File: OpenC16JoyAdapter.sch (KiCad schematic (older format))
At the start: 8 parts, among them J1 DB9_MALE, J2 TO_C16_MINI_DIN_8, SW1 PIN5_POWER, U1 74LS244

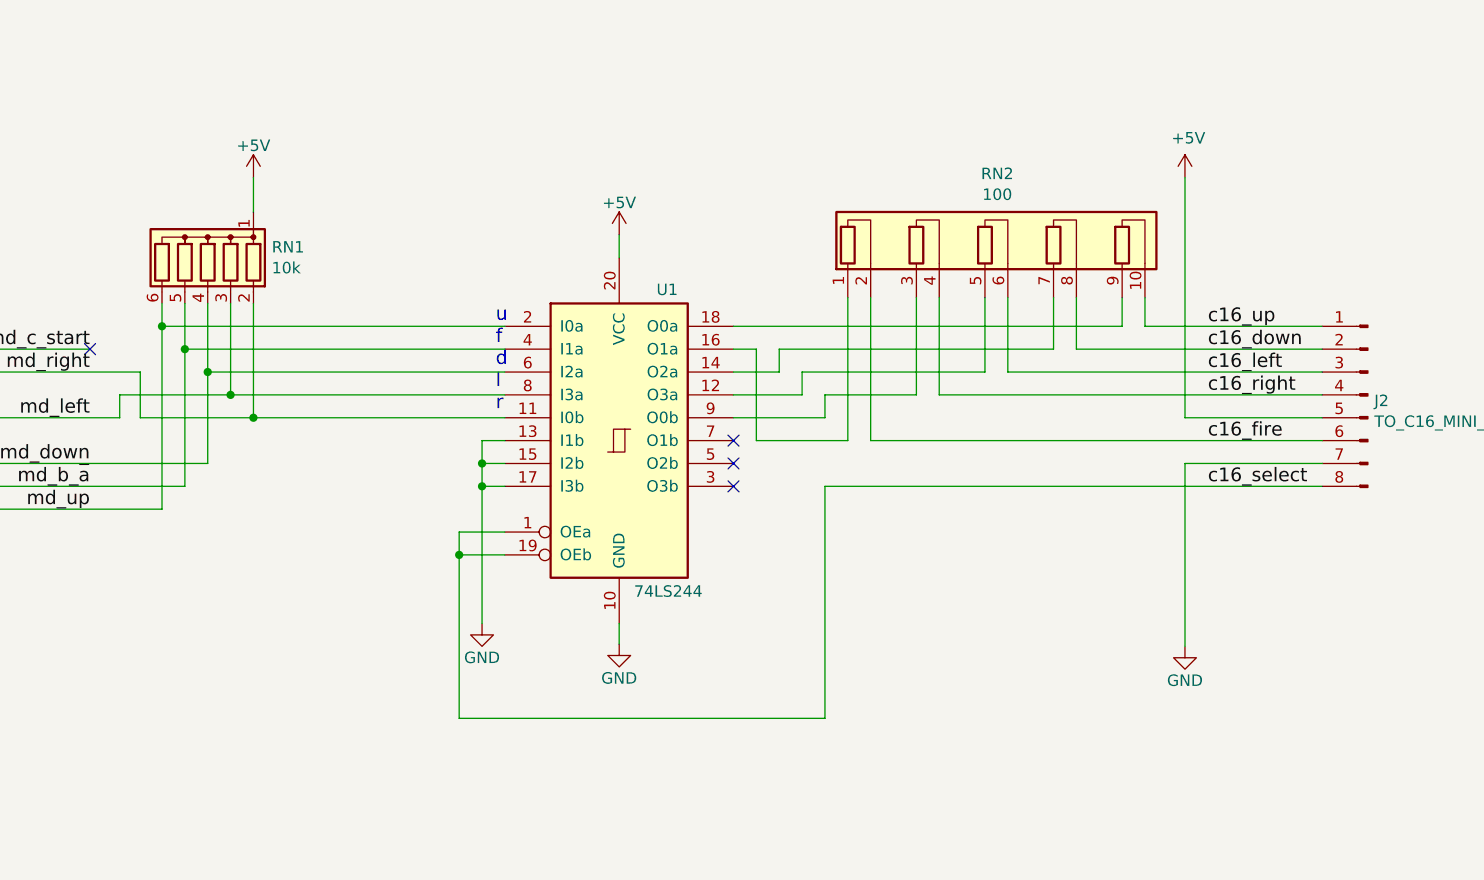
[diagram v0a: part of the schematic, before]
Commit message: Minor changes
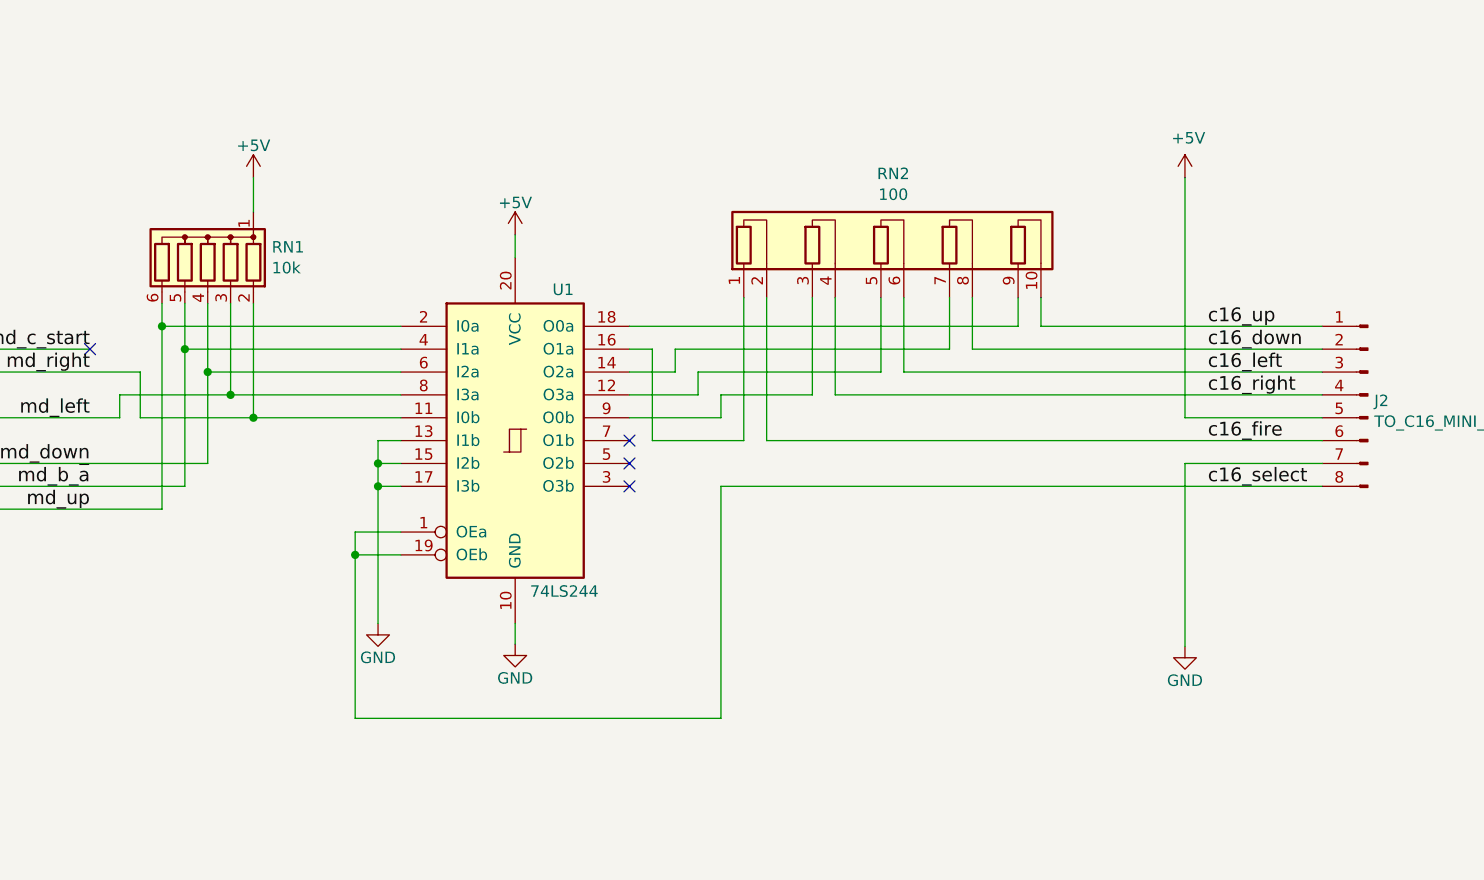
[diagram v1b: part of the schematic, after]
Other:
- note removed: "u\nf\nd\nl\nr"
- moved on the sheet: RN2, U1
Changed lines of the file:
@@
 Comp "SukkoPera"
 Comment1 "http://www.commodore.ca/manuals/funet/cbm/documents/projects/interfaces/plus4joy/plus4joy.html"
-Comment2 "Based on work by Levente Hársfalvi"
+Comment2 "Based on work by Levente Hársfalvi (TLC)"
 Comment3 "Licensed under CERN OHL v.1.2"
 Comment4 ""
@@
 L power:GND #PWR02
 U 1 1 5964022D
-P 4750 4600
-F 0 "#PWR02" H 4750 4350 50  0001 C CNN
-F 1 "GND" H 4750 4450 50  0000 C CNN
-F 2 "" H 4750 4600 50  0000 C CNN
-F 3 "" H 4750 4600 50  0000 C CNN
-	1    4750 4600
+P 4295 4600
+F 0 "#PWR02" H 4295 4350 50  0001 C CNN
+F 1 "GND" H 4295 4450 50  0000 C CNN
+F 2 "" H 4295 4600 50  0000 C CNN
+F 3 "" H 4295 4600 50  0000 C CNN
+	1    4295 4600
 	1    0    0    -1
 $EndComp
@@
 $EndComp
 Wire Wire Line
-	4750 3900 4850 3900
-Wire Wire Line
-	4650 4200 4850 4200
-Wire Wire Line
-	4650 4200 4650 4300
-Wire Wire Line
-	4850 4300 4650 4300
-Connection ~ 4650 4300
+	4295 3900 4395 3900
+Wire Wire Line
+	4195 4200 4395 4200
+Wire Wire Line
+	4195 4200 4195 4300
+Wire Wire Line
+	4395 4300 4195 4300
+Connection ~ 4195 4300
 Wire Wire Line
 	2460 2615 2460 2565
 Wire Wire Line
-	4750 3800 4850 3800
-Wire Wire Line
-	4750 3800 4750 3900
-Connection ~ 4750 3900
-Connection ~ 4750 4000
+	4295 3800 4395 3800
+Wire Wire Line
+	4295 3800 4295 3900
+Connection ~ 4295 3900
+Connection ~ 4295 4000
 Wire Wire Line
 	10375 3900 10375 3750
@@
 	3450 3200 3450 3400
 Wire Wire Line
-	4750 3900 4750 4000
-Wire Wire Line
-	4750 4000 4750 4600
-Wire Wire Line
-	4750 4000 4850 4000
-Wire Wire Line
-	3350 3300 4850 3300
-Wire Wire Line
-	3450 3400 4850 3400
+	4295 3900 4295 4000
+Wire Wire Line
+	4295 4000 4295 4600
+Wire Wire Line
+	4295 4000 4395 4000
+Wire Wire Line
+	3350 3300 4395 3300
+Wire Wire Line
+	3450 3400 4395 3400
 Wire Wire Line
 	3750 2650 3750 2800
@@
 $EndComp
 Wire Wire Line
-	6350 3800 6350 3175
-Wire Wire Line
-	6450 3800 6450 3175
-Wire Wire Line
-	6650 3600 6650 3175
-Wire Wire Line
-	6750 3600 6750 3175
-Wire Wire Line
-	6950 3500 6950 3175
-Wire Wire Line
-	7050 3500 7050 3175
-Wire Wire Line
-	7250 3400 6050 3400
-Wire Wire Line
-	7250 3175 7250 3400
-Wire Wire Line
-	7350 3175 7350 3400
-Wire Wire Line
-	7550 3300 7550 3175
-Wire Wire Line
-	7650 3175 7650 3300
-Wire Wire Line
-	5350 3000 5350 2900
-Wire Wire Line
-	5950 3800 6350 3800
-Wire Wire Line
-	5950 3400 5950 3800
-Wire Wire Line
-	5850 3400 5950 3400
-Wire Wire Line
-	6250 3600 6650 3600
-Wire Wire Line
-	6250 3600 6250 3700
-Wire Wire Line
-	6250 3700 5850 3700
-Wire Wire Line
-	6150 3500 6950 3500
-Wire Wire Line
-	6150 3600 6150 3500
-Wire Wire Line
-	5850 3600 6150 3600
-Wire Wire Line
-	6050 3500 6050 3400
-Wire Wire Line
-	5850 3500 6050 3500
-Wire Wire Line
-	5850 3300 7550 3300
-Wire Wire Line
-	6250 4000 8425 4000
+	5895 3800 5895 3175
+Wire Wire Line
+	5995 3800 5995 3175
+Wire Wire Line
+	6195 3600 6195 3175
+Wire Wire Line
+	6295 3600 6295 3175
+Wire Wire Line
+	6495 3500 6495 3175
+Wire Wire Line
+	6595 3500 6595 3175
+Wire Wire Line
+	6795 3400 5595 3400
+Wire Wire Line
+	6795 3175 6795 3400
+Wire Wire Line
+	6895 3175 6895 3400
+Wire Wire Line
+	7095 3300 7095 3175
+Wire Wire Line
+	7195 3175 7195 3300
+Wire Wire Line
+	4895 3000 4895 2900
+Wire Wire Line
+	5495 3800 5895 3800
+Wire Wire Line
+	5495 3400 5495 3800
+Wire Wire Line
+	5395 3400 5495 3400
+Wire Wire Line
+	5795 3600 6195 3600
+Wire Wire Line
+	5795 3600 5795 3700
+Wire Wire Line
+	5795 3700 5395 3700
+Wire Wire Line
+	5695 3500 6495 3500
+Wire Wire Line
+	5695 3600 5695 3500
+Wire Wire Line
+	5395 3600 5695 3600
+Wire Wire Line
+	5595 3500 5595 3400
+Wire Wire Line
+	5395 3500 5595 3500
+Wire Wire Line
+	5395 3300 7095 3300
+Wire Wire Line
+	5795 4000 8425 4000
 Wire Wire Line
 	7825 3900 7825 4700
@@
 	8425 3900 7825 3900
 Wire Wire Line
-	6450 3800 8425 3800
+	5995 3800 8425 3800
 Wire Wire Line
 	7825 3700 7825 2650
@@
 	8425 3700 7825 3700
 Wire Wire Line
-	6750 3600 8425 3600
-Wire Wire Line
-	7050 3500 8425 3500
-Wire Wire Line
-	7350 3400 8425 3400
-Wire Wire Line
-	7650 3300 8425 3300
+	6295 3600 8425 3600
+Wire Wire Line
+	6595 3500 8425 3500
+Wire Wire Line
+	6895 3400 8425 3400
+Wire Wire Line
+	7195 3300 8425 3300
 $Comp
 L power:+5V #PWR08
 U 1 1 596A3F1E
-P 5350 2900
-F 0 "#PWR08" H 5350 2750 50  0001 C CNN
-F 1 "+5V" H 5350 3040 50  0000 C CNN
-F 2 "" H 5350 2900 50  0000 C CNN
-F 3 "" H 5350 2900 50  0000 C CNN
-	1    5350 2900
-	1    0    0    -1
-$EndComp
-NoConn ~ 5850 4000
-NoConn ~ 5850 3900
-NoConn ~ 5850 3800
+P 4895 2900
+F 0 "#PWR08" H 4895 2750 50  0001 C CNN
+F 1 "+5V" H 4895 3040 50  0000 C CNN
+F 2 "" H 4895 2900 50  0000 C CNN
+F 3 "" H 4895 2900 50  0000 C CNN
+	1    4895 2900
+	1    0    0    -1
+$EndComp
+NoConn ~ 5395 4000
+NoConn ~ 5395 3900
+NoConn ~ 5395 3800
 Text Label 7925 4000 0    60   ~ 0
 c16_select
@@
 L 74xx:74LS244 U1
 U 1 1 65B63CCD
-P 5350 3800
-F 0 "U1" H 5560 4460 50  0000 C CNN
-F 1 "74LS244" H 5565 3140 50  0000 C CNN
-F 2 "Package_DIP:DIP-20_W7.62mm_Socket_LongPads" H 5350 3800 50  0001 C CNN
-F 3 "http://www.ti.com/lit/ds/symlink/sn74ls244.pdf" H 5350 3800 50  0001 C CNN
-	1    5350 3800
-	1    0    0    -1
-$EndComp
-Wire Wire Line
-	5350 4600 5350 4690
+P 4895 3800
+F 0 "U1" H 5105 4460 50  0000 C CNN
+F 1 "74LS244" H 5110 3140 50  0000 C CNN
+F 2 "Package_DIP:DIP-20_W7.62mm_Socket_LongPads" H 4895 3800 50  0001 C CNN
+F 3 "http://www.ti.com/lit/ds/symlink/sn74ls244.pdf" H 4895 3800 50  0001 C CNN
+	1    4895 3800
+	1    0    0    -1
+$EndComp
+Wire Wire Line
+	4895 4600 4895 4690
 $Comp
 L power:GND #PWR0103
 U 1 1 65B8FAC7
-P 5350 4690
-F 0 "#PWR0103" H 5350 4440 50  0001 C CNN
-F 1 "GND" H 5350 4540 50  0000 C CNN
-F 2 "" H 5350 4690 50  0000 C CNN
-F 3 "" H 5350 4690 50  0000 C CNN
-	1    5350 4690
-	1    0    0    -1
-$EndComp
-Wire Wire Line
-	4650 5015 6250 5015
-Wire Wire Line
-	4650 4300 4650 5015
-Wire Wire Line
-	6250 4000 6250 5015
+P 4895 4690
+F 0 "#PWR0103" H 4895 4440 50  0001 C CNN
+F 1 "GND" H 4895 4540 50  0000 C CNN
+F 2 "" H 4895 4690 50  0000 C CNN
+F 3 "" H 4895 4690 50  0000 C CNN
+	1    4895 4690
+	1    0    0    -1
+$EndComp
+Wire Wire Line
+	4195 5015 5795 5015
+Wire Wire Line
+	4195 4300 4195 5015
+Wire Wire Line
+	5795 4000 5795 5015
 $Comp
 L power:+5V #PWR0104
@@
 L Device:R_Pack05_SIP RN2
 U 1 1 65B9ACA3
-P 6950 2975
-F 0 "RN2" H 7004 3317 50  0000 C CNN
-F 1 "100" H 7004 3226 50  0000 C CNN
-F 2 "Resistor_THT:R_Array_SIP10" V 7825 2975 50  0001 C CNN
-F 3 "http://www.vishay.com/docs/31509/csc.pdf" H 6950 2975 50  0001 C CNN
-	1    6950 2975
+P 6495 2975
+F 0 "RN2" H 6549 3317 50  0000 C CNN
+F 1 "100" H 6549 3226 50  0000 C CNN
+F 2 "Resistor_THT:R_Array_SIP10" V 7370 2975 50  0001 C CNN
+F 3 "http://www.vishay.com/docs/31509/csc.pdf" H 6495 2975 50  0001 C CNN
+	1    6495 2975
 	1    0    0    -1
 $EndComp
@@
 Wire Wire Line
 	2335 3500 3255 3500
-Text Notes 4810 3675 0    60   ~ 0
-u\nf\nd\nl\nr
 Wire Wire Line
 	2335 3700 3165 3700
@@
 	2335 3900 3550 3900
 Wire Wire Line
-	4850 3500 3550 3500
+	4395 3500 3550 3500
 Connection ~ 3550 3500
 Wire Wire Line
@@
 Connection ~ 3650 3600
 Wire Wire Line
-	3650 3600 4850 3600
-Wire Wire Line
-	3750 3700 4850 3700
+	3650 3600 4395 3600
+Wire Wire Line
+	3750 3700 4395 3700
 Wire Wire Line
 	3650 3600 3165 3600
